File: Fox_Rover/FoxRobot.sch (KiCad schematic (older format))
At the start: 34 parts, among them J1 Screw_Terminal_01x02, J2 XT60-M_Green, J3 XT60-M_Red, J4 Screw_Terminal_01x02, J5 Conn_02x10_Odd_Even, J6 Screw_Terminal_01x02, J7 Conn_02x10_Odd_Even, K1 40.52.7.012.0000, K2 G2RK-1_12DC, K3 ADJH23005, K4 ADJH23005, Q1 BS170, Q2 BS170, Q3 BS170, Q4 BS170, Q5 BS170, Q6 BS170, Q7 BS170, Q8 BS170, Q9 BS170, U1 JCL3024S05

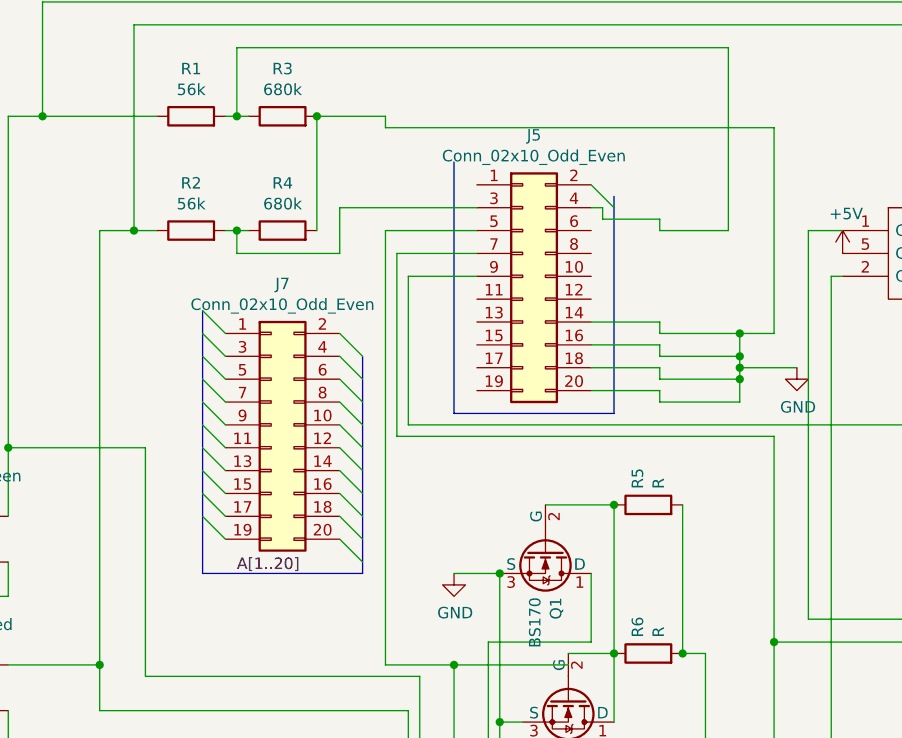
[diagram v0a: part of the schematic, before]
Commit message: PCB design suitable
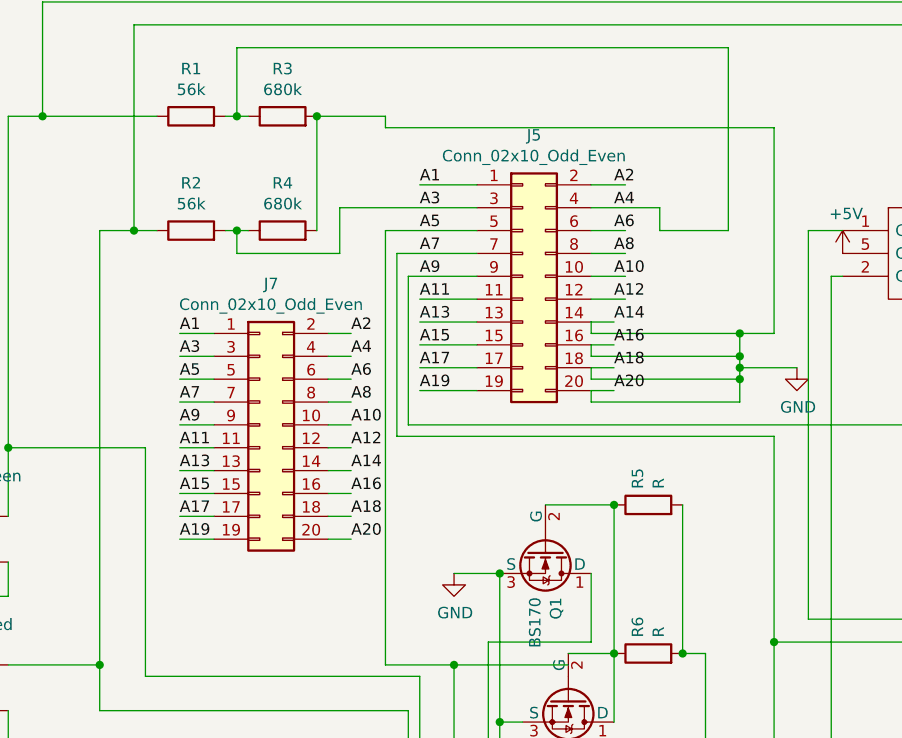
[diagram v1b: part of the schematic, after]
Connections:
- net labels added: A1, A10, A11, A12, A13, A14, A15, A16, A17, A18, A19, A2, A20, A3, A4, A5, A6, A7, A8, A9
- net labels removed: A[1..20]
- wire segments 207 -> 236
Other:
- moved on the sheet: J7
